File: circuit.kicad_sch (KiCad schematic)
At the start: 70 parts, among them J1 1725656, J2 CTX 3V3 GND TX, J3 CRX 3V3 GND RX, J4 PICO GP4/GP5 CAN, J5 2171750001, Q1 PMV100EPAR, U1 SN65HVD230DR, U2 AMS1117-3.3_C347222

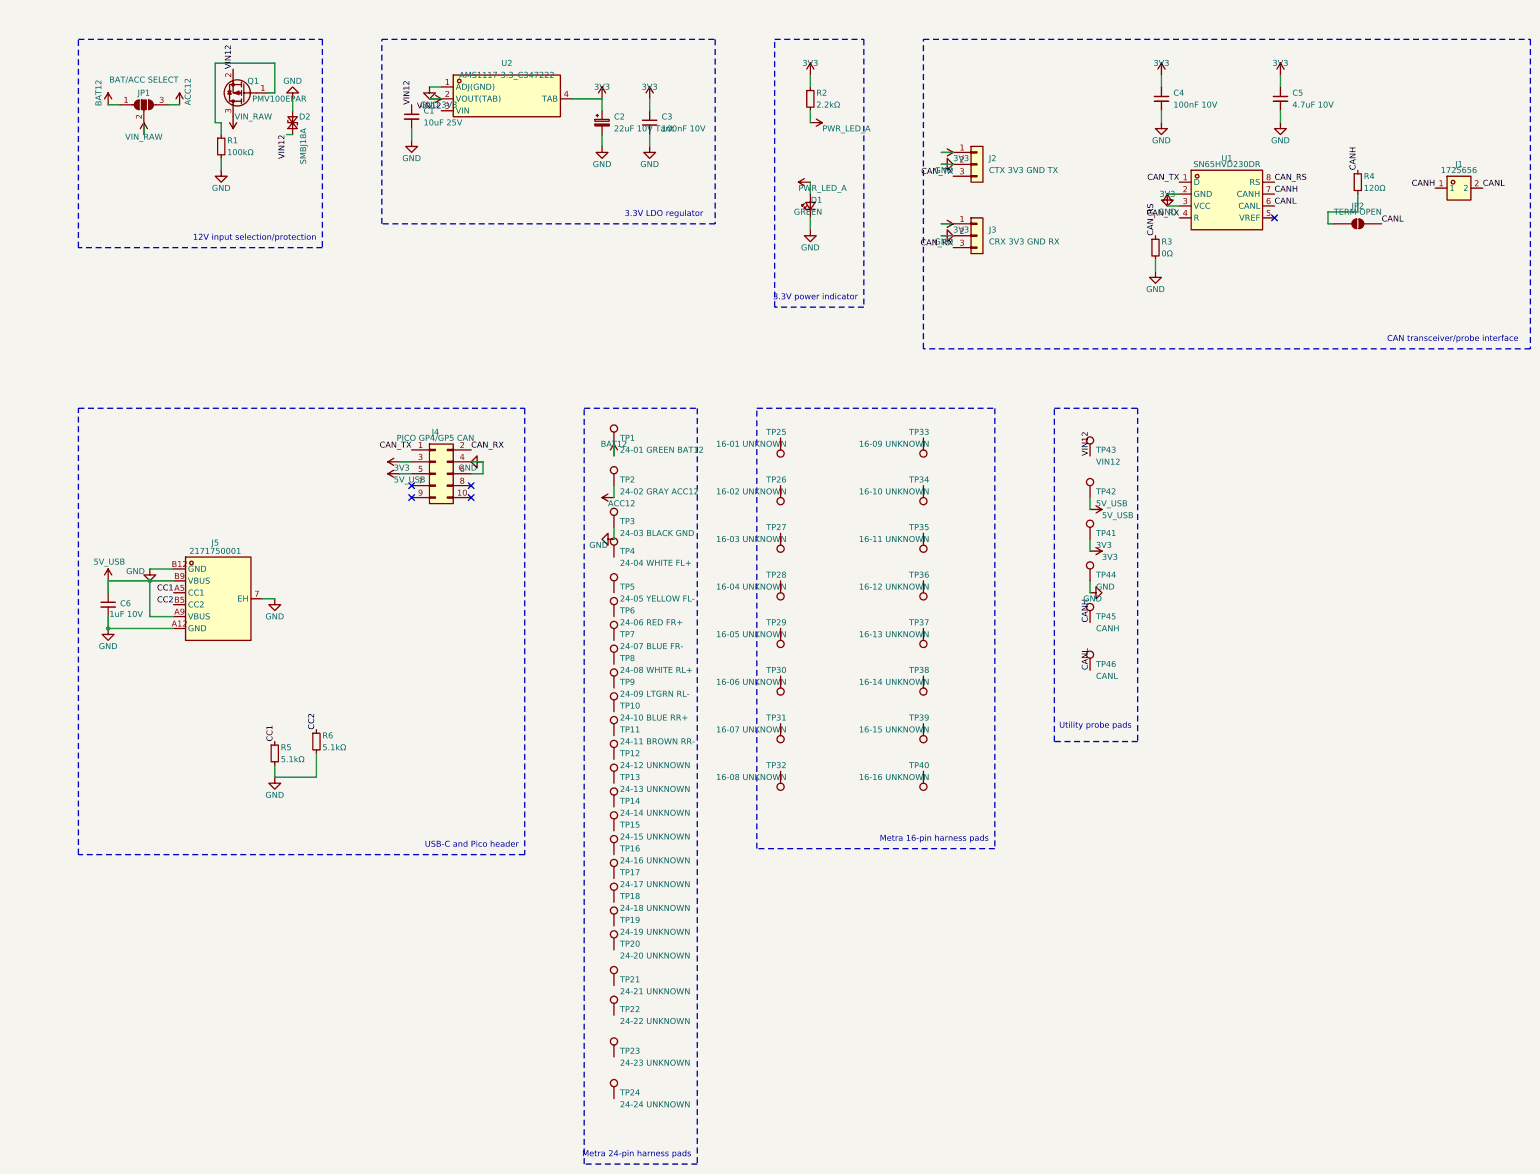
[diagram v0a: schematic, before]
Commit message: (karl) updates
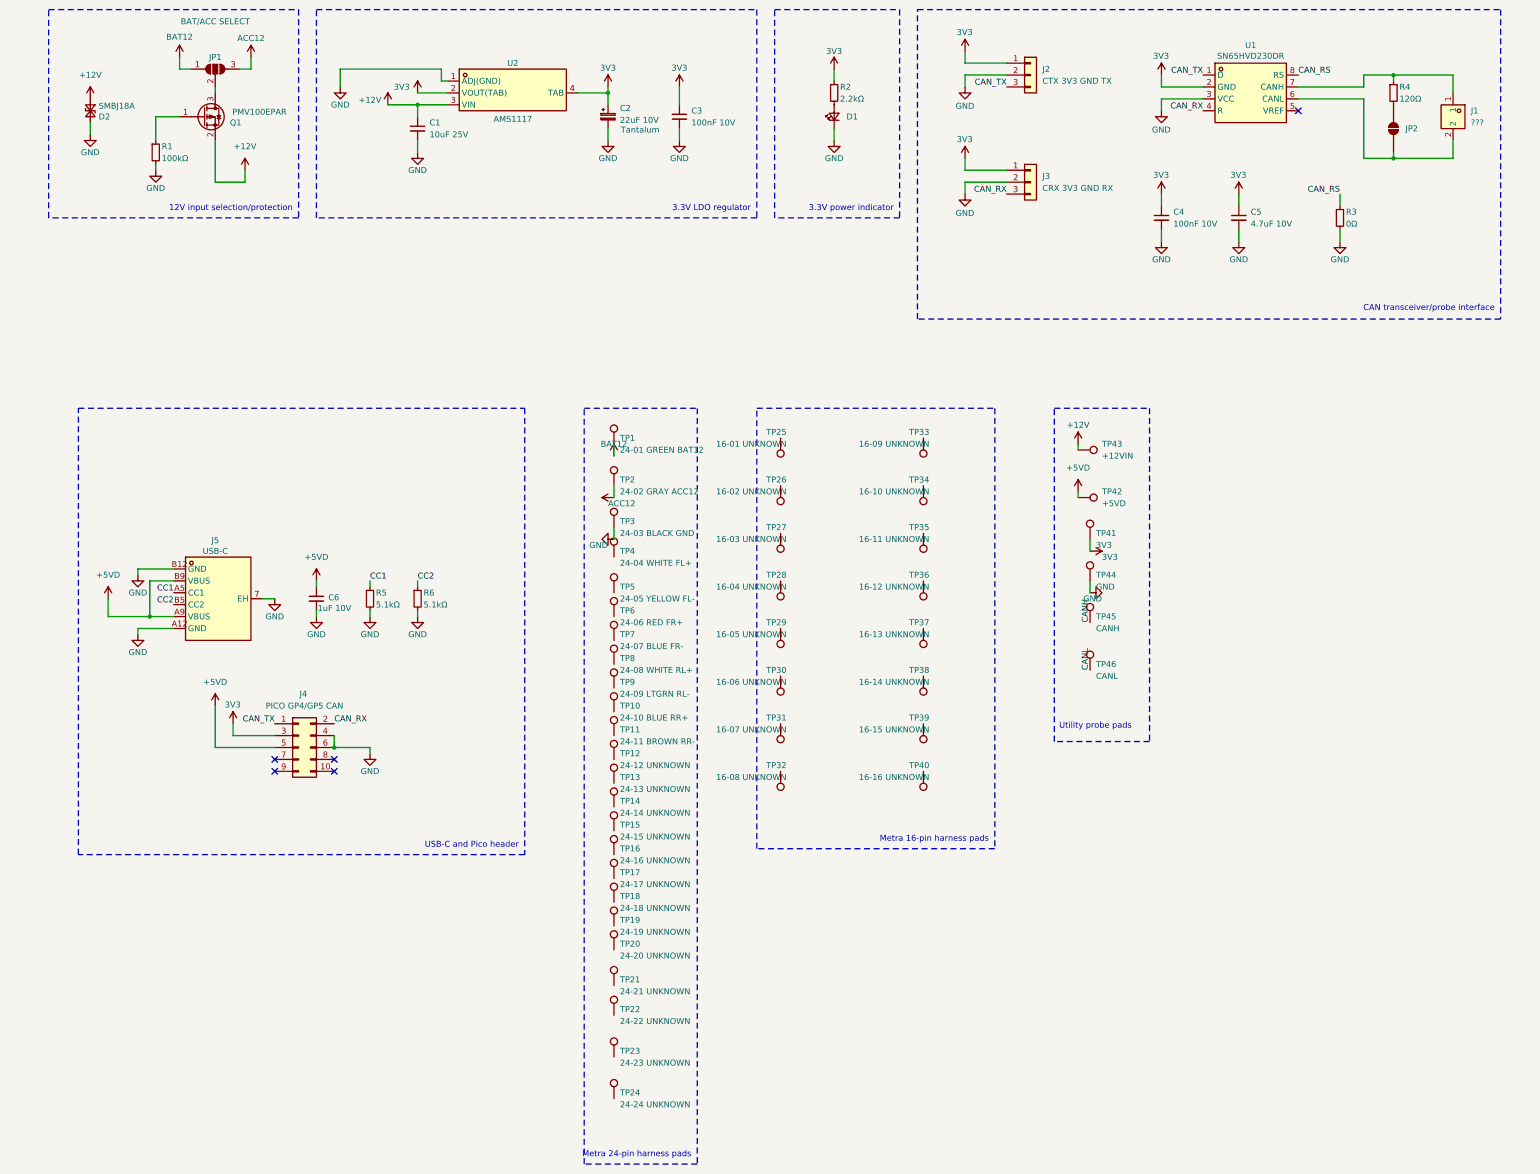
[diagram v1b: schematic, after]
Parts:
- C2: value 22uF 10V Tant -> 22uF 10V
- D1: value GREEN -> Green LED
- J1: value 1725656 -> ???
- J5: value 2171750001 -> USB-C
- TP42: value 5V_USB -> +5VD
- TP43: value VIN12 -> +12VIN
- U2: value AMS1117-3.3_C347222 -> AMS1117
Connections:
- net 3V3: now also U1.2 (GND); no longer U1.3 (VCC)
- net CANH: no longer J1.1, R4.1, U1.7 (CANH)
- net CANL: no longer J1.2, JP2.2 (B), U1.6 (CANL)
- net GND: now also U1.3 (VCC); no longer U1.2 (GND)
- net at JP2.1 (A): now also J1.2, U1.6 (CANL); no longer R4.2
- net 5V_USB renamed +5VD
- net PWR_LED_A: no longer names the net of D1.2 (A), R2.2
- net VIN12 renamed +12V
- net VIN_RAW: no longer names the net of JP1.2 (C), Q1.3 (D)
- new net: J1.1, R4.1, U1.7 (CANH)
- new net: JP2.2 (B), R4.2
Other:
- moved on the sheet: C1, C2, C3, C4, C5, D1, D2, J1, J2, J3, J4, JP1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

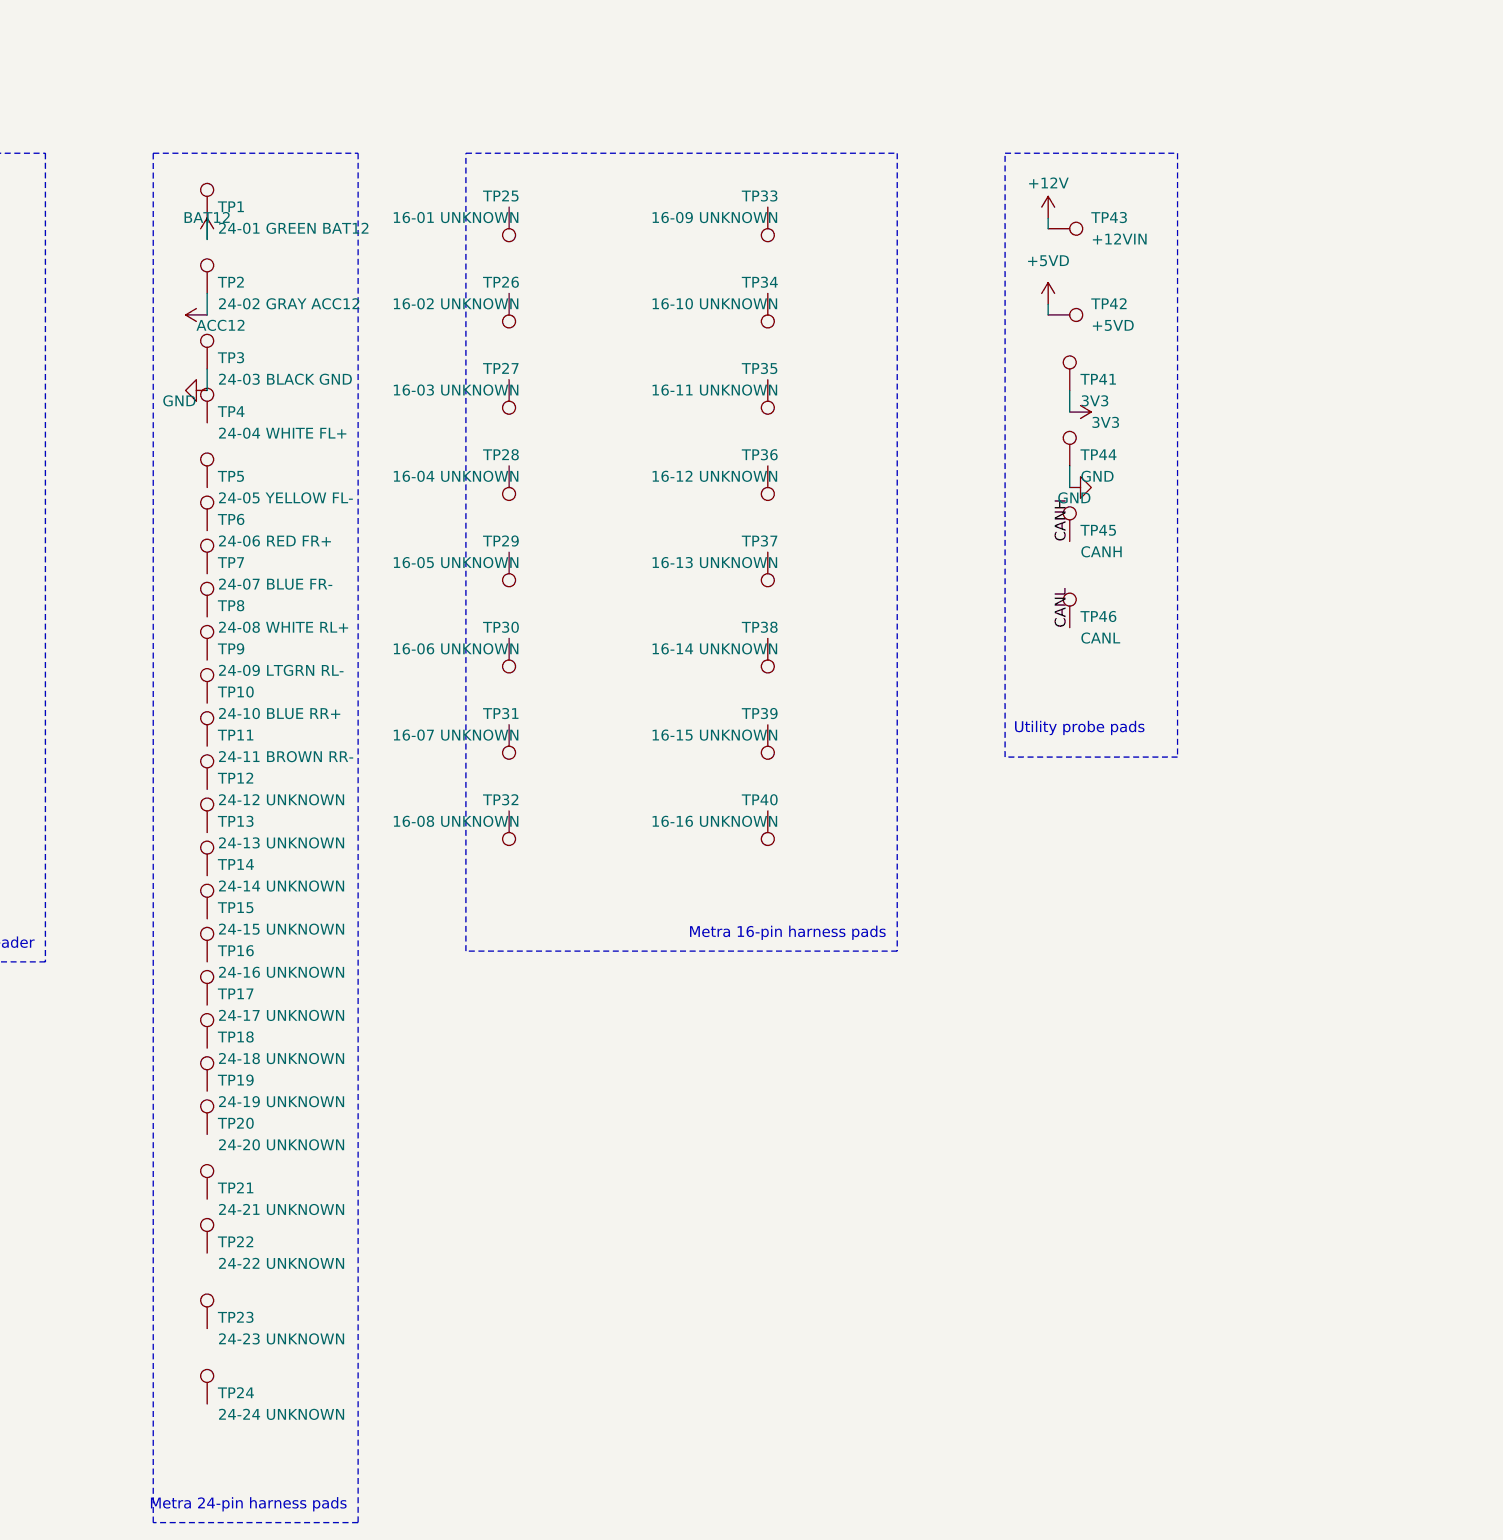
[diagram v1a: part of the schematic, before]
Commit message: small updates
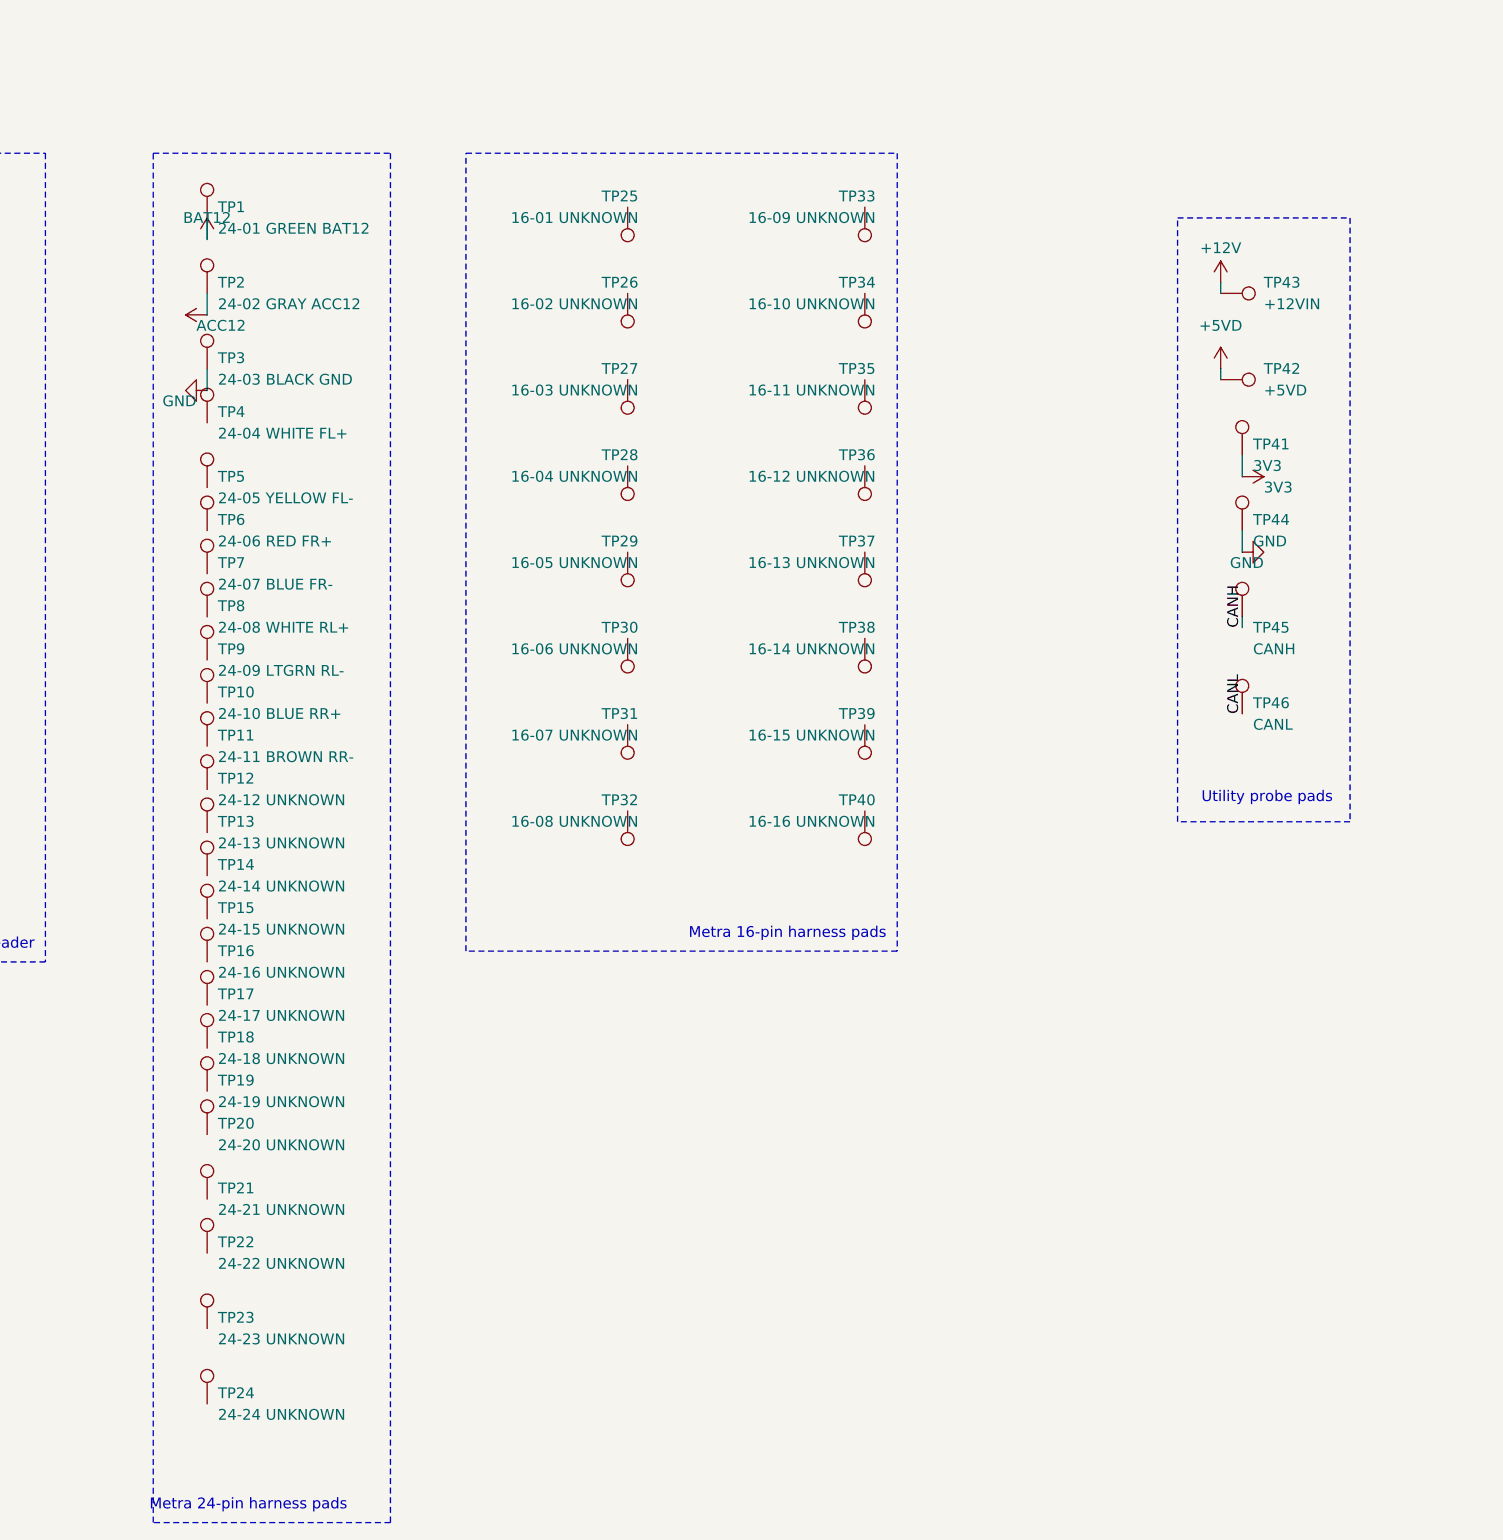
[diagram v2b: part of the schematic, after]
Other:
- company: (none) -> Jasper Mayone
- title: (none) -> Mazzy Harness Probe
- moved on the sheet: TP25, TP26, TP27, TP28, TP29, TP30, TP31, TP32, TP33, TP34, TP35, TP36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
